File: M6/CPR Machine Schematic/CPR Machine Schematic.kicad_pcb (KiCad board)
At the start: 2 copper layers, 79.8 x 63 mm, 85 parts, among them J1 Battery 22.2V IN, J10 Laser Port, J11 Raspberry_Pi_2_3, J2 Power Switch, J3 GND Spare Headers, J4 +V Spare Headers, J5 Conn_02x20_Odd_Even, J6 I2C Port, J7 Stop Button Port, J8 Go Button Port, J9 Force Sensor, Q1 DMMT5401 PNP, Q2 SSM3J332R, Q3 DMG2305UX-EV, Q4 DMMT5401 PNP, Q5 T2N7002BK,LM, Q6 T2N7002BK,LM, Q7 T2N7002BK,LM, U1 3.3V Buck, U2 12V Buck, U3 MAX42403AFLB+, U4 MCP6004, U5 MCP3021A5T-E_OT

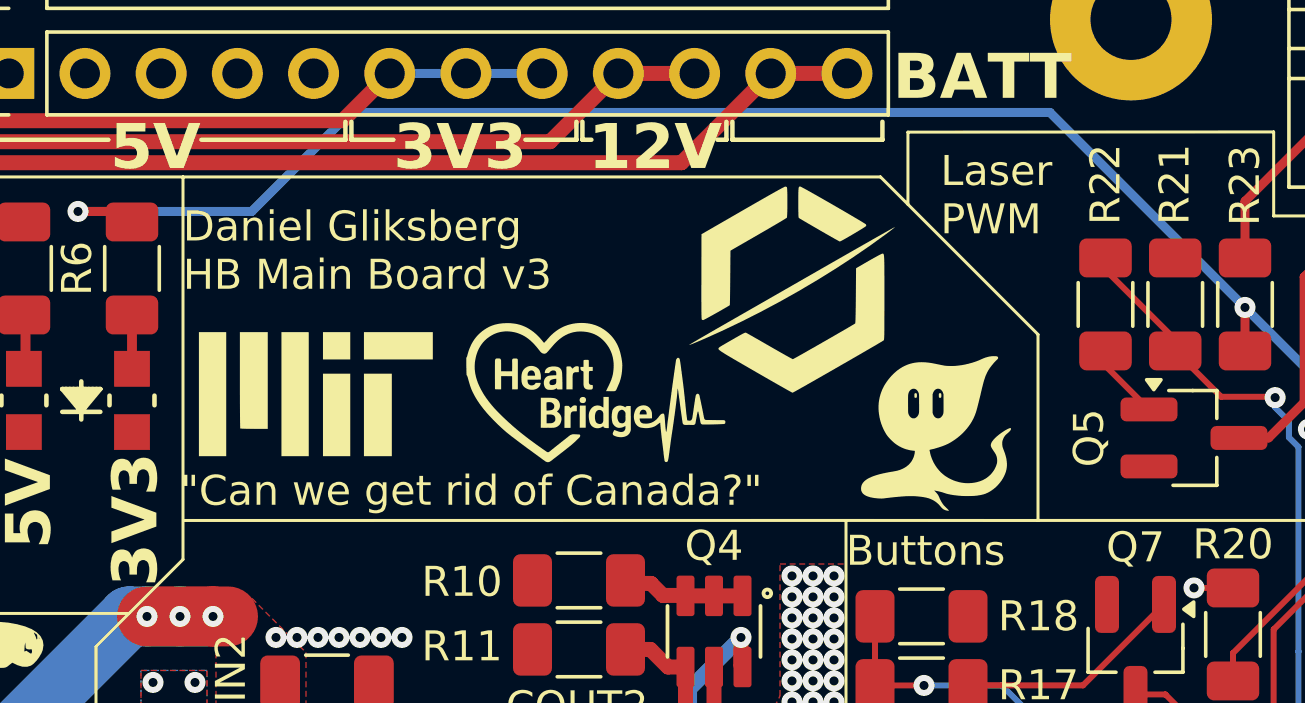
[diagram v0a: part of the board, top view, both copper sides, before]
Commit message: Prod files for V3
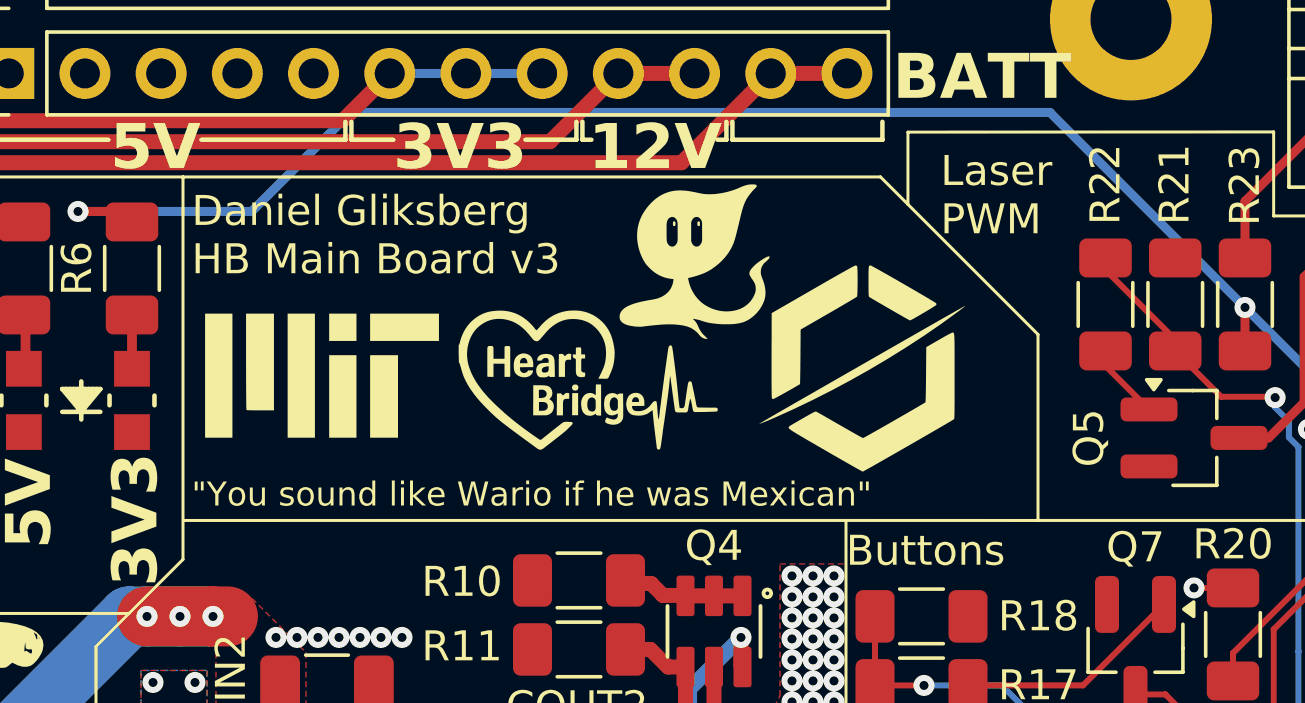
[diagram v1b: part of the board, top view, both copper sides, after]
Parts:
- moved G***2 9.88 mm to (162.1, 84.1)
- moved G***3 3.52 mm to (167.6, 87.6)
- moved G***1 0.65 mm to (149.6, 87.9)
- moved REF**2 0.49 mm to (158.5, 87.9)
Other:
- board text added: "{dblquote}You sound like Wario if he was Mexican{dblquote}"
- board text removed: "{dblquote}Can we get rid of Canada?{dblquote}"
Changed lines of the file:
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@@
 	(footprint "Images:MIT"
 		(layer "F.Cu")
-		(at 149.4 88.5)
+		(at 149.606 87.884)
 		(property "Reference" "G***1"
 			(at 0 0 0)
@@
 	(footprint "Images:LilGuy"
 		(layer "F.Cu")
-		(at 170.1 89.8)
+		(at 162.052 84.074)
 		(property "Reference" "G***2"
 			(at 0 0 0)
@@
 	(footprint "MAX42402AFLB_:Untitled"
 		(layer "F.Cu")
-		(at 158.75 88.3)
+		(at 158.496 87.884)
 		(property "Reference" "REF**2"
 			(at 0 -0.5 0)
@@
 	(footprint "Images:Occam"
 		(layer "F.Cu")
-		(at 165.3 85)
+		(at 167.64 87.63)
 		(property "Reference" "G***3"
 			(at 0 0 0)
@@
 	)
 	(gr_text "Daniel Gliksberg\nHB Main Board v3"
-		(at 145 85.1 0)
+		(at 145.288 84.582 0)
 		(layer "F.SilkS")
 		(effects
@@
 		)
 	)
-	(gr_text "{dblquote}Can we get rid of Canada?{dblquote}"
-		(at 144.9 92.3 0)
+	(gr_text "{dblquote}You sound like Wario if he was Mexican{dblquote}"
+		(at 145.288 92.3 0)
 		(layer "F.SilkS")
 		(effects
 			(font
-				(size 1 1)
+				(size 0.8 0.8)
 				(thickness 0.15)
 			)
